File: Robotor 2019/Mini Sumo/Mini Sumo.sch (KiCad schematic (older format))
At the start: 72 parts, among them J1 Conn_01x03_Male, J2 Conn_01x04_Female, J3 USB_B_Mini, J4 Conn_01x01, J5 Conn_01x02, J6 Conn_01x01, M1 Motor_DC, M2 Motor_DC, SW1 SW_Push, SW2 SW_Push, U1 AMS1117-3V3, U2 VNH7100BA, U3 L78L05_SOT89, U4 STM32F103C8Tx, U5 VNH7100BA, Y1 32.768Khz, Y2 8Mhz

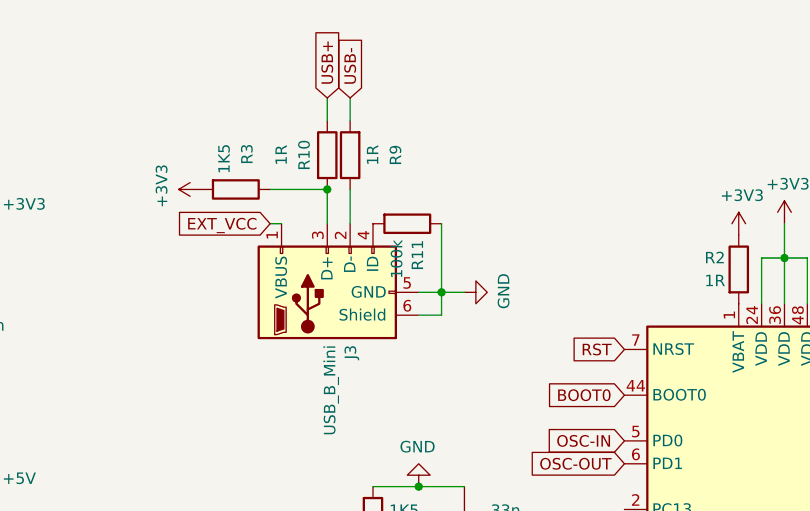
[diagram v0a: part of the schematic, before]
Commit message: Honestly I don't even remember
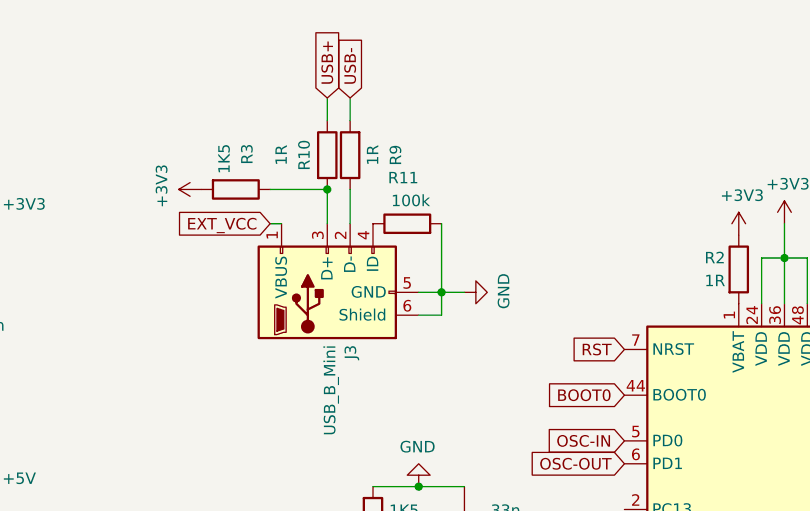
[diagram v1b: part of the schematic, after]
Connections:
- net GND: now also R11.2; no longer R11.1
- net at J3.4 (ID): now also R11.1; no longer R11.2
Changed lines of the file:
@@
 U 1 1 5D397BF9
 P 4050 1400
-F 0 "R11" H 4120 1446 50  0000 L CNN
-F 1 "100k" H 4120 1355 50  0000 L CNN
+F 0 "R11" V 4250 1350 50  0000 L CNN
+F 1 "100k" V 4150 1300 50  0000 L CNN
 F 2 "Resistor_SMD:R_0805_2012Metric_Pad1.15x1.40mm_HandSolder" V 3980 1400 50  0001 C CNN
 F 3 "~" H 4050 1400 50  0001 C CNN
 	1    4050 1400
-	0    1    1    0
+	0    -1   -1   0
 $EndComp
 Wire Wire Line

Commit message: Fecking Stuff
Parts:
- U2, U5: symbol Driver_Motor:VNH7100BA -> Mini-Sumo-rescue:VNH7100BA-Driver_Motor
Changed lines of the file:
@@
 $EndComp
 $Comp
-L Driver_Motor:VNH7100BA U5
+L Mini-Sumo-rescue:VNH7100BA-Driver_Motor U5
 U 1 1 5D58D0DD
 P 9250 5400
@@
 $EndComp
 $Comp
-L Driver_Motor:VNH7100BA U2
+L Mini-Sumo-rescue:VNH7100BA-Driver_Motor U2
 U 1 1 5D5DE765
 P 9250 3900
